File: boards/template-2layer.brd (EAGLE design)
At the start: 34.3 x 27.9 mm, 26 parts, among them U2 XBEE-1B3, U3 V_REG_LDOSMD

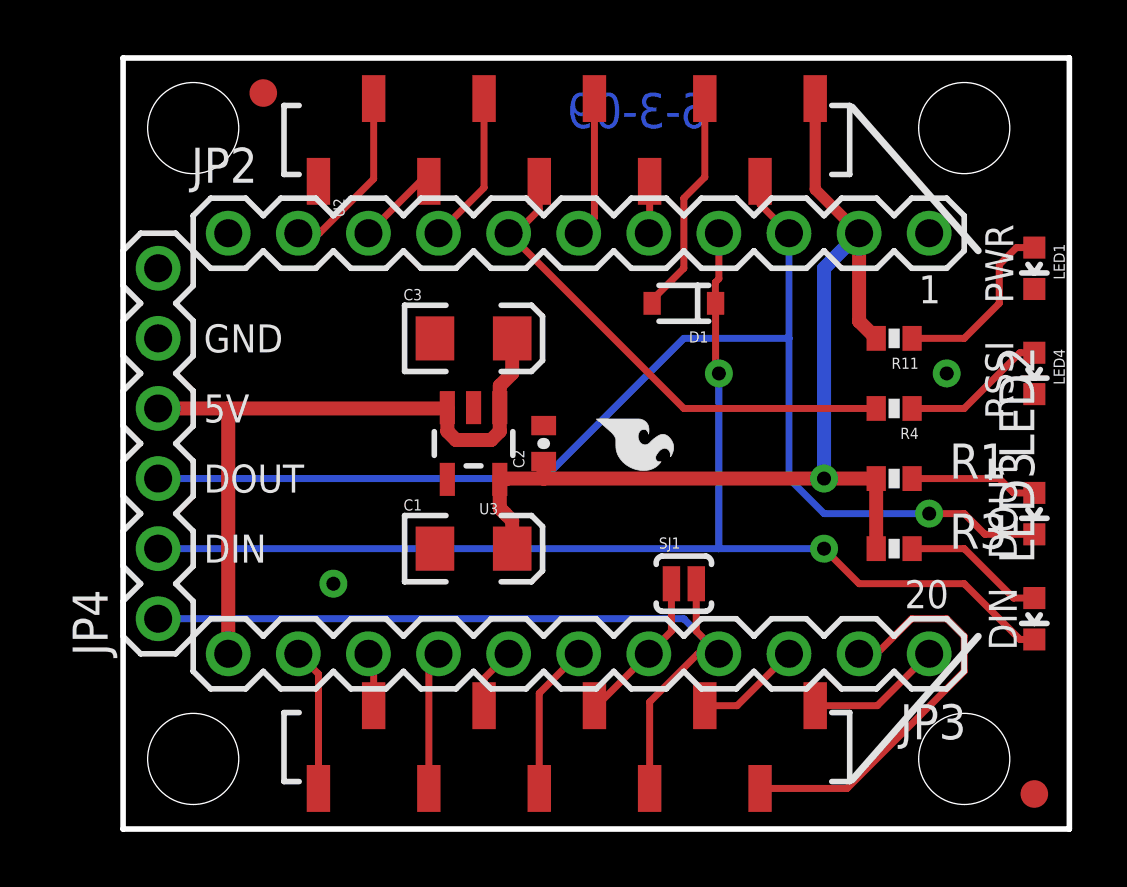
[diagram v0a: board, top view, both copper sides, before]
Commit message: cleaned up template
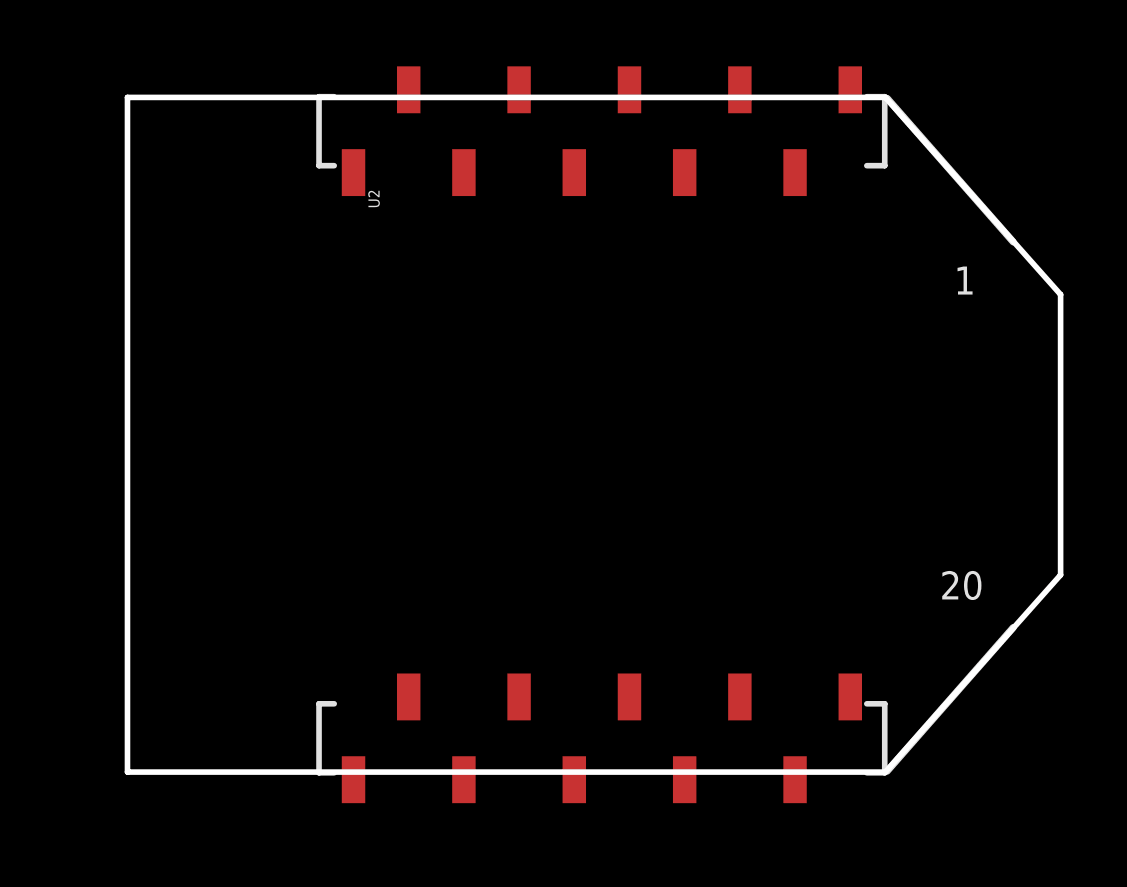
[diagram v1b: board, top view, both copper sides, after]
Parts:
- removed C1, C3: 10uF, SparkFun:EIA3216
- removed C2: 0.1uF, SparkFun:0402-CAP
- removed D1: (no value), SparkFun:SOD-323
- removed JP2, JP3: M11PTH, SparkFun:1X11
- removed JP4: (no value), SparkFun:1X06
- removed LED1, LED2: Red, SparkFun:LED-0603
- removed LED3, LED4: Green, SparkFun:LED-0603
- removed R1, R11, R3, R4: 1K, SparkFun:0402-RES
- removed SJ1: SOLDERJUMPERNO, SparkFun:SJ_2S-NO
- removed U$1: LOGO-SFESK, SparkFun:SFE-LOGO-FLAME
- removed U$10, U$11, U$5, U$9: STAND-OFF, SparkFun:STAND-OFF
- removed U$16, U$7: FIDUCIAL1X2, SparkFun:FIDUCIAL-1X2
- removed U$4: LOGO-SFENEW, SparkFun:SFE-NEW-WEBLOGO
- removed U3: V_REG_LDOSMD, SparkFun:SOT23-5
- moved U2 1.31 mm to (6.35, 14.3)
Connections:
- removed net 5V: C3.A, JP3.11, JP4.4, U3.1, U3.3
- removed net DIN: D1.1, JP2.8, JP4.2, LED3.C
- removed net N$1: LED2.A, R1.2
- removed net N$2: LED4.A, R4.1
- removed net N$3: D1.2, U2.3
- removed net N$38: LED1.A, R11.1
- removed net N$4: LED3.A, R3.2
- net 3.3V: no longer C1.A, C2.1, JP2.10, R1.1, R11.2, R3.1, U3.5
- net CTS: no longer JP3.9
- net DIO0: no longer JP3.1
- net DIO1: no longer JP3.2
- net DIO11: no longer JP2.4
- net DIO12: no longer JP2.7
- net DIO2: no longer JP3.3
- net DIO3: no longer JP3.4, JP4.1, SJ1.2
- net DIO4: no longer JP3.10
- net DIO5: no longer JP3.6
- net DIO9: no longer JP3.8
- net DOUT: no longer JP2.9, JP4.3, LED2.C
- net DTR: no longer JP2.2
- net GND: no longer C1.C, C2.2, C3.C, JP2.1, JP2.11, JP4.5, JP4.6, LED1.C, LED4.C, U3.2
- net RES1: no longer JP2.3
- net RES2: no longer JP3.7
- net RESET: no longer JP2.6
- net RSSI: no longer JP2.5, R4.2
- net RTS: no longer JP3.5, SJ1.1
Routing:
- net DOUT: track 45.9 -> 0.00 mm, vias 1 -> 0
- net DIN: track 44.7 -> 0.00 mm, vias 2 -> 0
- net 3.3V: track 39.0 -> 0.00 mm, vias 1 -> 0
- net DIO3: track 30.1 -> 0.00 mm
- net 5V: track 26.0 -> 0.00 mm
- net RSSI: track 18.4 -> 0.00 mm
- net DIO1: track 15.0 -> 0.00 mm
- net N$3: track 8.38 -> 0.00 mm
- net N$38: track 6.61 -> 0.00 mm
- net DTR: track 6.46 -> 0.00 mm
- net RTS: track 5.63 -> 0.00 mm
- net DIO11: track 5.56 -> 0.00 mm
- net DIO5: track 5.47 -> 0.00 mm
- net N$2: track 5.27 -> 0.00 mm
- net DIO4: track 5.18 -> 0.00 mm
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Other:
- board size 34.3 x 27.9 mm -> 33.8 x 24.4 mm
- board text removed: "6-3-09"
- board text removed: "PWR"
